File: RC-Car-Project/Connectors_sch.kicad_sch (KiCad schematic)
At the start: 19 parts, among them J1 Conn_01x02_Pin, J10 ANT_IF, J11 Conn_01x02, J12 Conn_01x02, J13 RF_IF, J14 2171790001, J2 Conn_01x02_Pin, J3 Conn_01x02_Pin, J4 Conn_01x02_Pin, J5 MCU_IF, J6 Conn_01x02, J7 Conn_01x02, J8 Conn_01x02, J9 Conn_02x09_Odd_Even, U4 USBLC6-2SC6

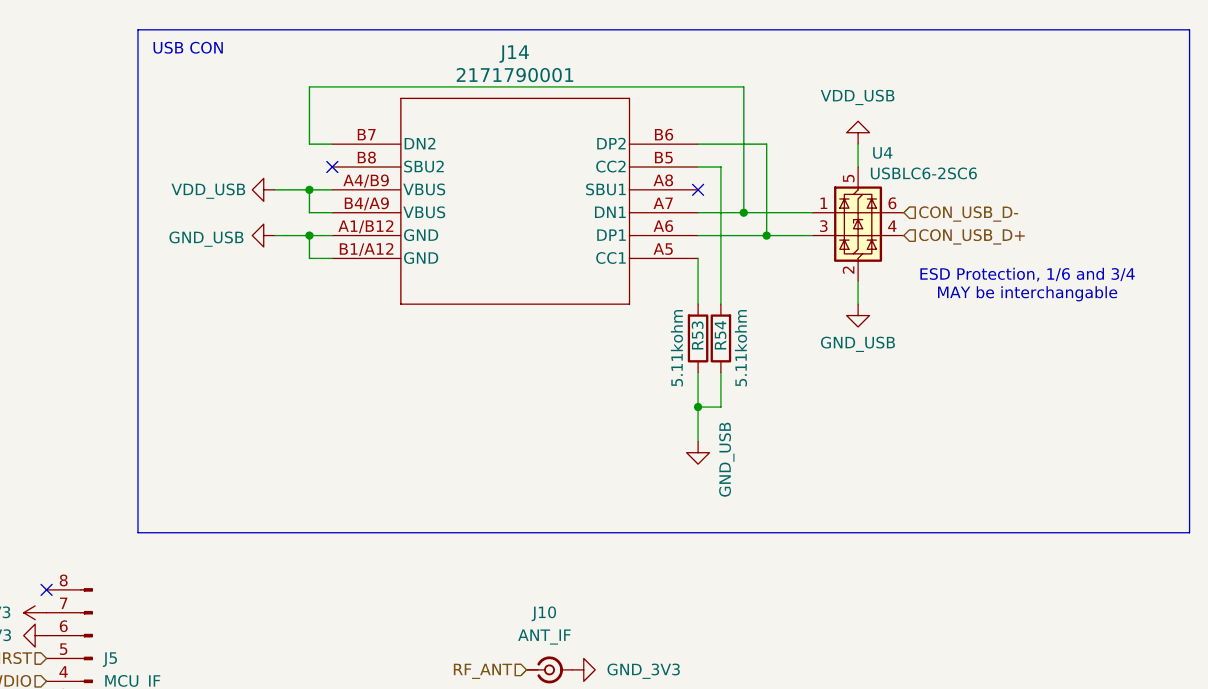
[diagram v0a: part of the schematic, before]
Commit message: I'm tired boss
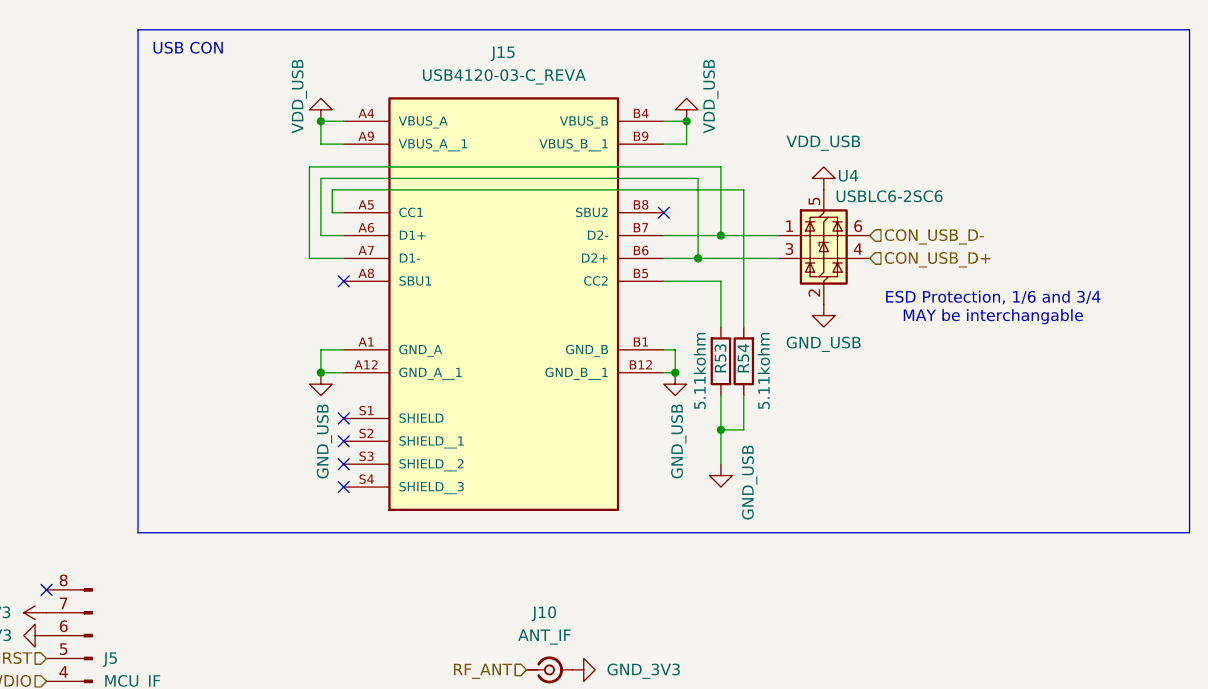
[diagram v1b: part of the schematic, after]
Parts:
- removed J14: 2171790001, USB-C 2171790001:2171790001_MOL, symbol USB-C 2171790001:2171790001
- added J15: USB4120-03-C_REVA, USB4120-03-C:GCT_USB4120-03-C_REVA, symbol USB4120-03-C:USB4120-03-C_REVA
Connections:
- net GND_USB: now also J15.A1 (GND_A), J15.A12 (GND_A__1), J15.B1 (GND_B), J15.B12 (GND_B__1)
- net VDD_USB: now also J15.A4 (VBUS_A), J15.A9 (VBUS_A__1), J15.B4 (VBUS_B), J15.B9 (VBUS_B__1)
- net at R53.2: now also J15.B5 (CC2)
- net at U4.3 (I/O2): now also J15.A6 (D1+), J15.B6 (D2+)
- net at U4.1 (I/O1): now also J15.A7 (D1-), J15.B7 (D2-)
- net at R54.2: now also J15.A5 (CC1)
- no-connect marks 3 -> 7
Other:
- moved on the sheet: R53, R54, U4
